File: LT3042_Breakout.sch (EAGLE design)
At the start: 2 parts, among them IC1 LT3042, J1 XR2A-0811-N

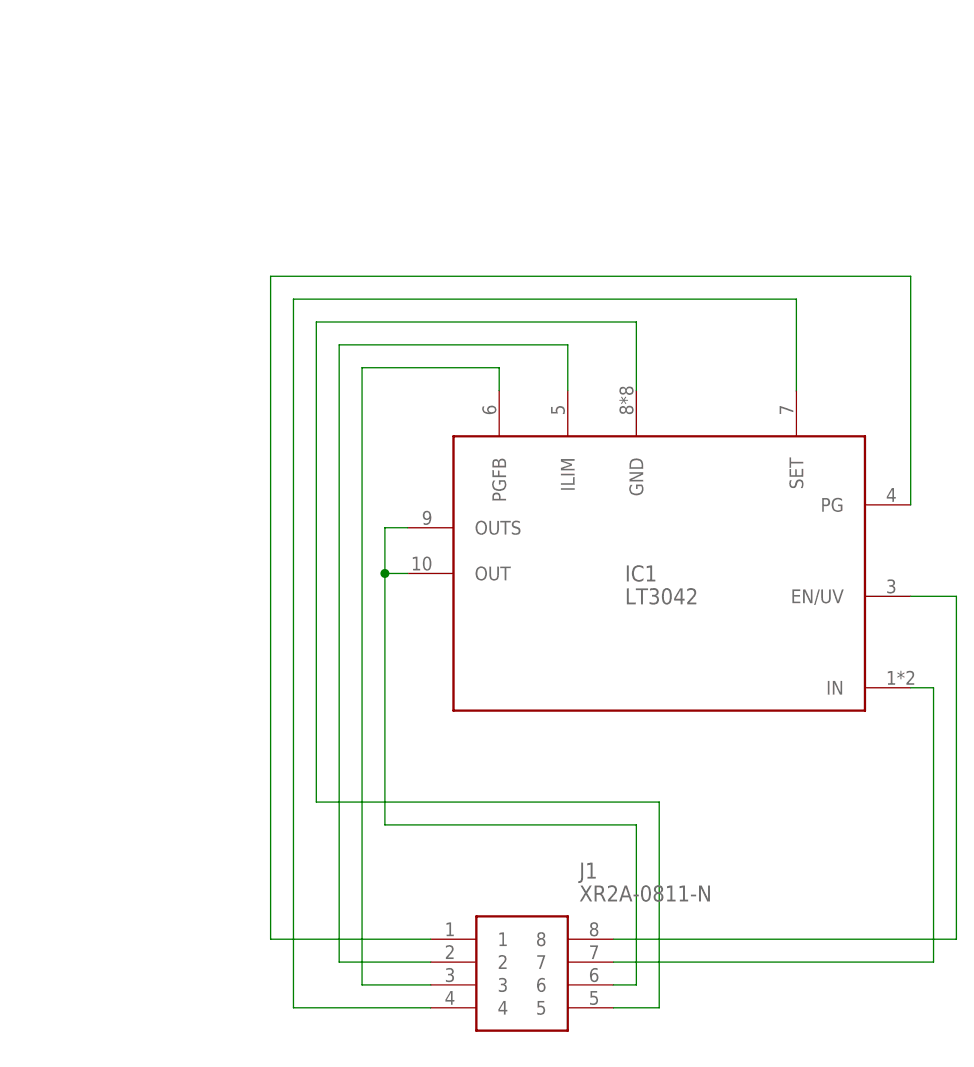
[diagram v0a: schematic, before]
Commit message: Redid LT3042 breakout
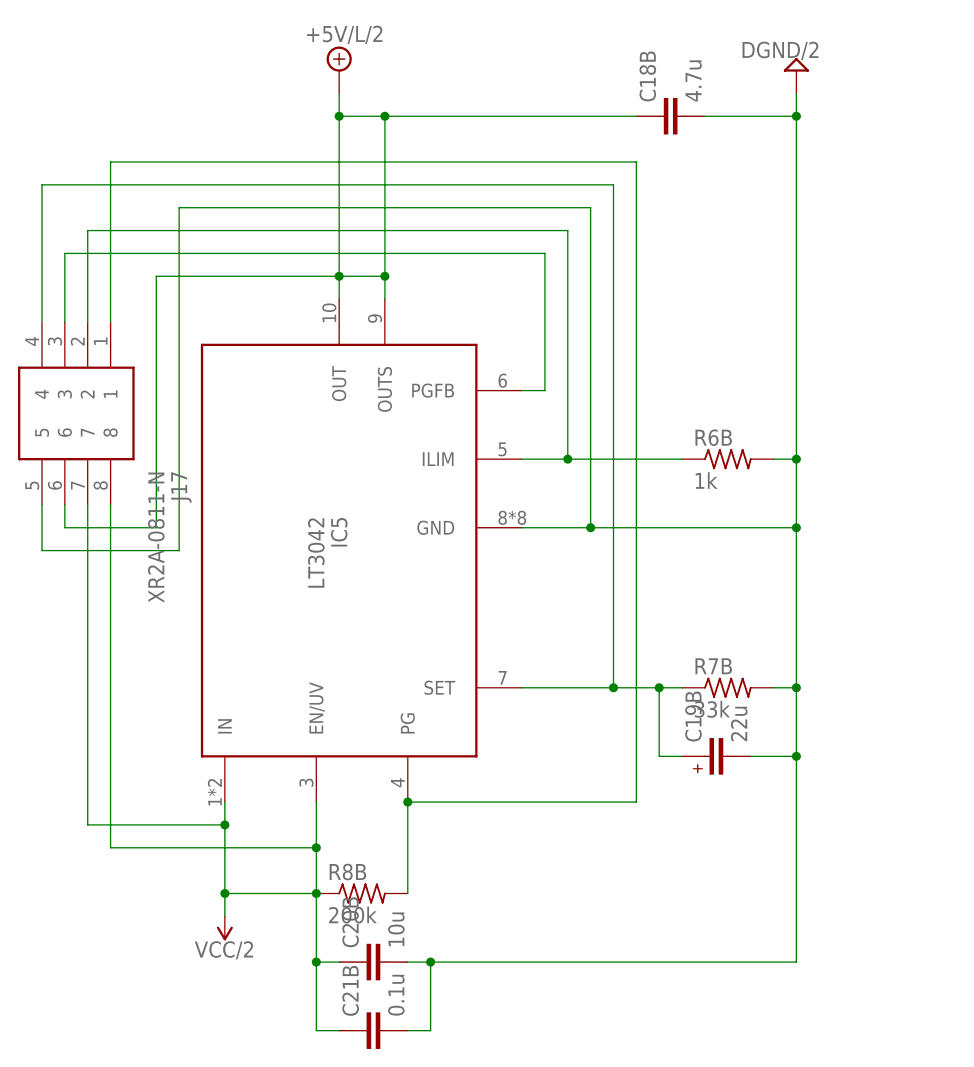
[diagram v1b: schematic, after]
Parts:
- removed IC1: LT3042, Dual Mono Amp Library:LT3042
- removed J1: XR2A-0811-N, XR2A-0811-N:XR2A-0811-N
- added C18B: 4.7u, Dual Mono Amp Library:EMK212ABJ475KG-T
- added C19B: 22u, Dual Mono Amp Library:EMK316BB7226ML-T
- added C20B: 10u, Dual Mono Amp Library:EMK212BB7106KG-T
- added C21B: 0.1u, Dual Mono Amp Library:EMF212B7104KGHT
- added IC5: LT3042, Dual Mono Amp Library:LT3042
- added J17: XR2A-0811-N, XR2A-0811-N:XR2A-0811-N
- added R6B: 1k, Dual Mono Amp Library:CHP0805-FX-1001ELF
- added R7B: 33k, Dual Mono Amp Library:CPF0805B51KE1
- added R8B: 200k, Dual Mono Amp Library:RR1220P-204-D
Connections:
- removed net N$1: IC1.IN, J1.7
- removed net N$2: IC1.EN/UV, J1.8
- removed net N$3: IC1.PG, J1.1
- removed net N$4: IC1.ILIM, J1.2
- removed net N$5: IC1.OUT, IC1.OUTS, J1.6
- removed net N$6: IC1.GND, J1.5
- removed net N$7: IC1.SET, J1.4
- removed net N$8: IC1.PGFB, J1.3
- new net +5V/L/2: C18B.1, IC5.OUT, IC5.OUTS, J17.6
- new net DGND/2: C18B.2, C19B.2, C20B.2, C21B.2, IC5.GND, J17.5, R6B.2, R7B.2
- new net N$103: C19B.1, IC5.SET, J17.4, R7B.1
- new net N$46: IC5.PG, J17.1, R8B.2
- new net N$47: IC5.ILIM, J17.2, R6B.1
- new net N$48: IC5.PGFB, J17.3
- new net VCC/2: C20B.1, C21B.1, IC5.EN/UV, IC5.IN, J17.7, J17.8, R8B.1
